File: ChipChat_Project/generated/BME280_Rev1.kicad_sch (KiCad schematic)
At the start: 0 parts

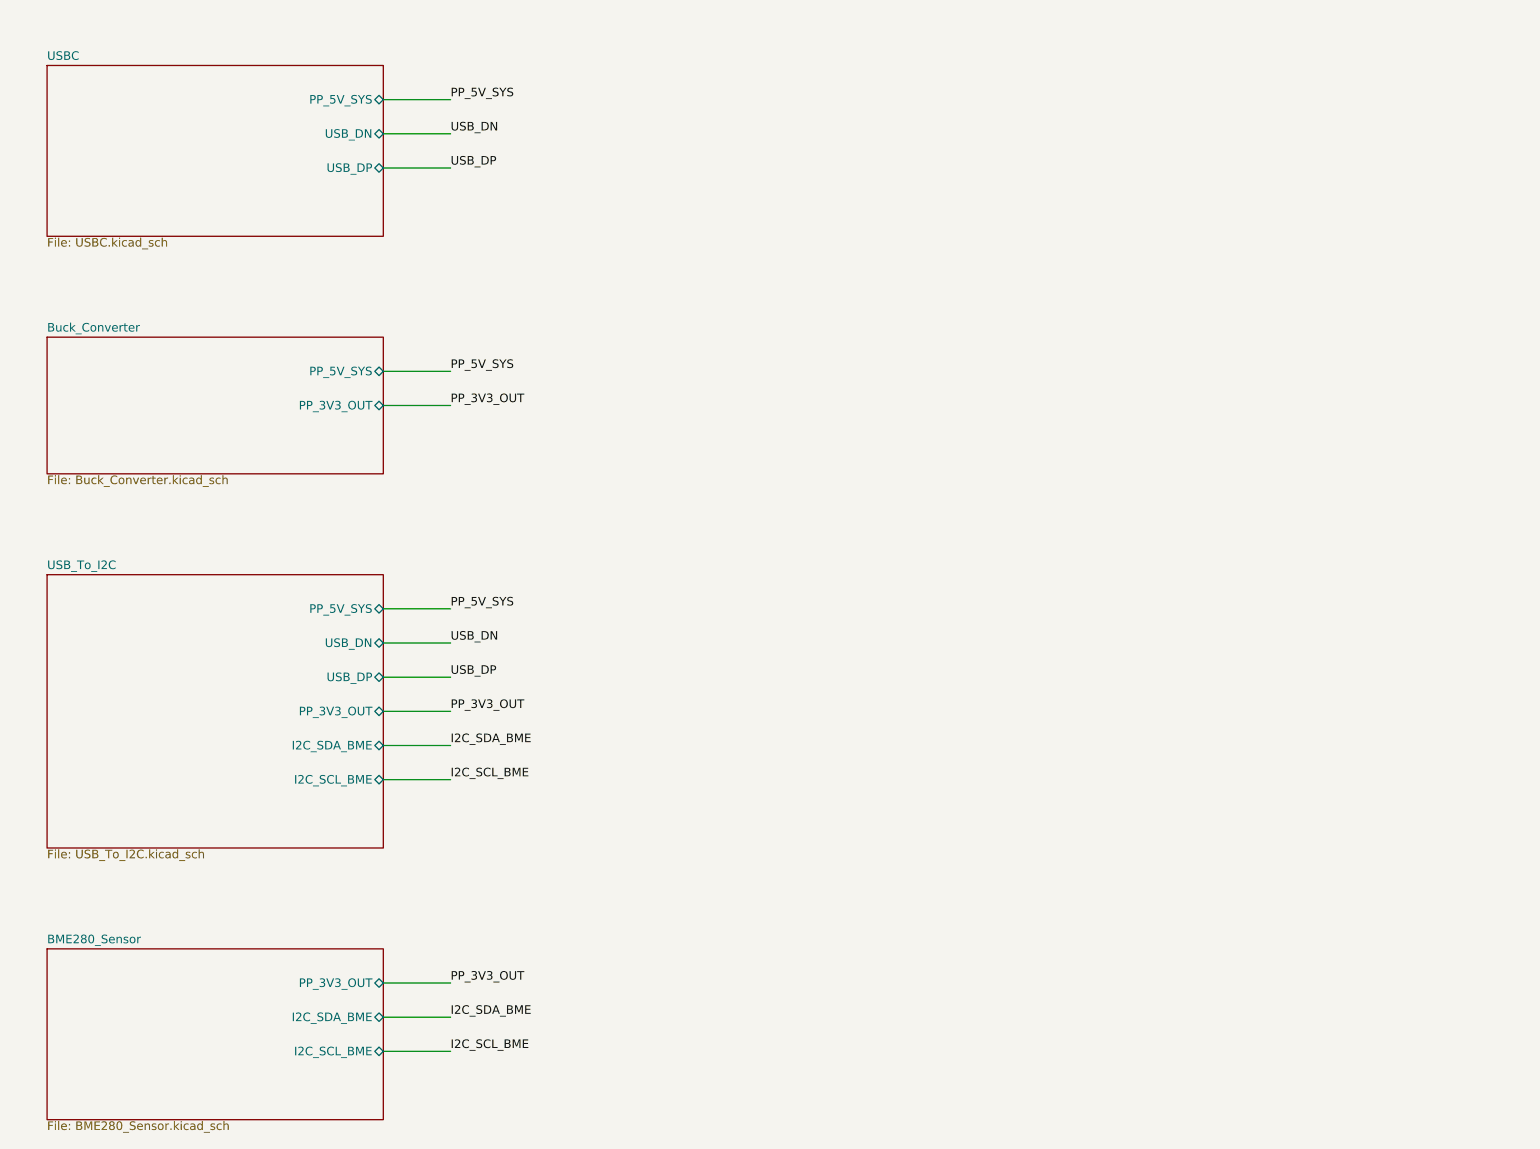
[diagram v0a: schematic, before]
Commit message: 💾 snapshot 2026-02-23_00-19-22
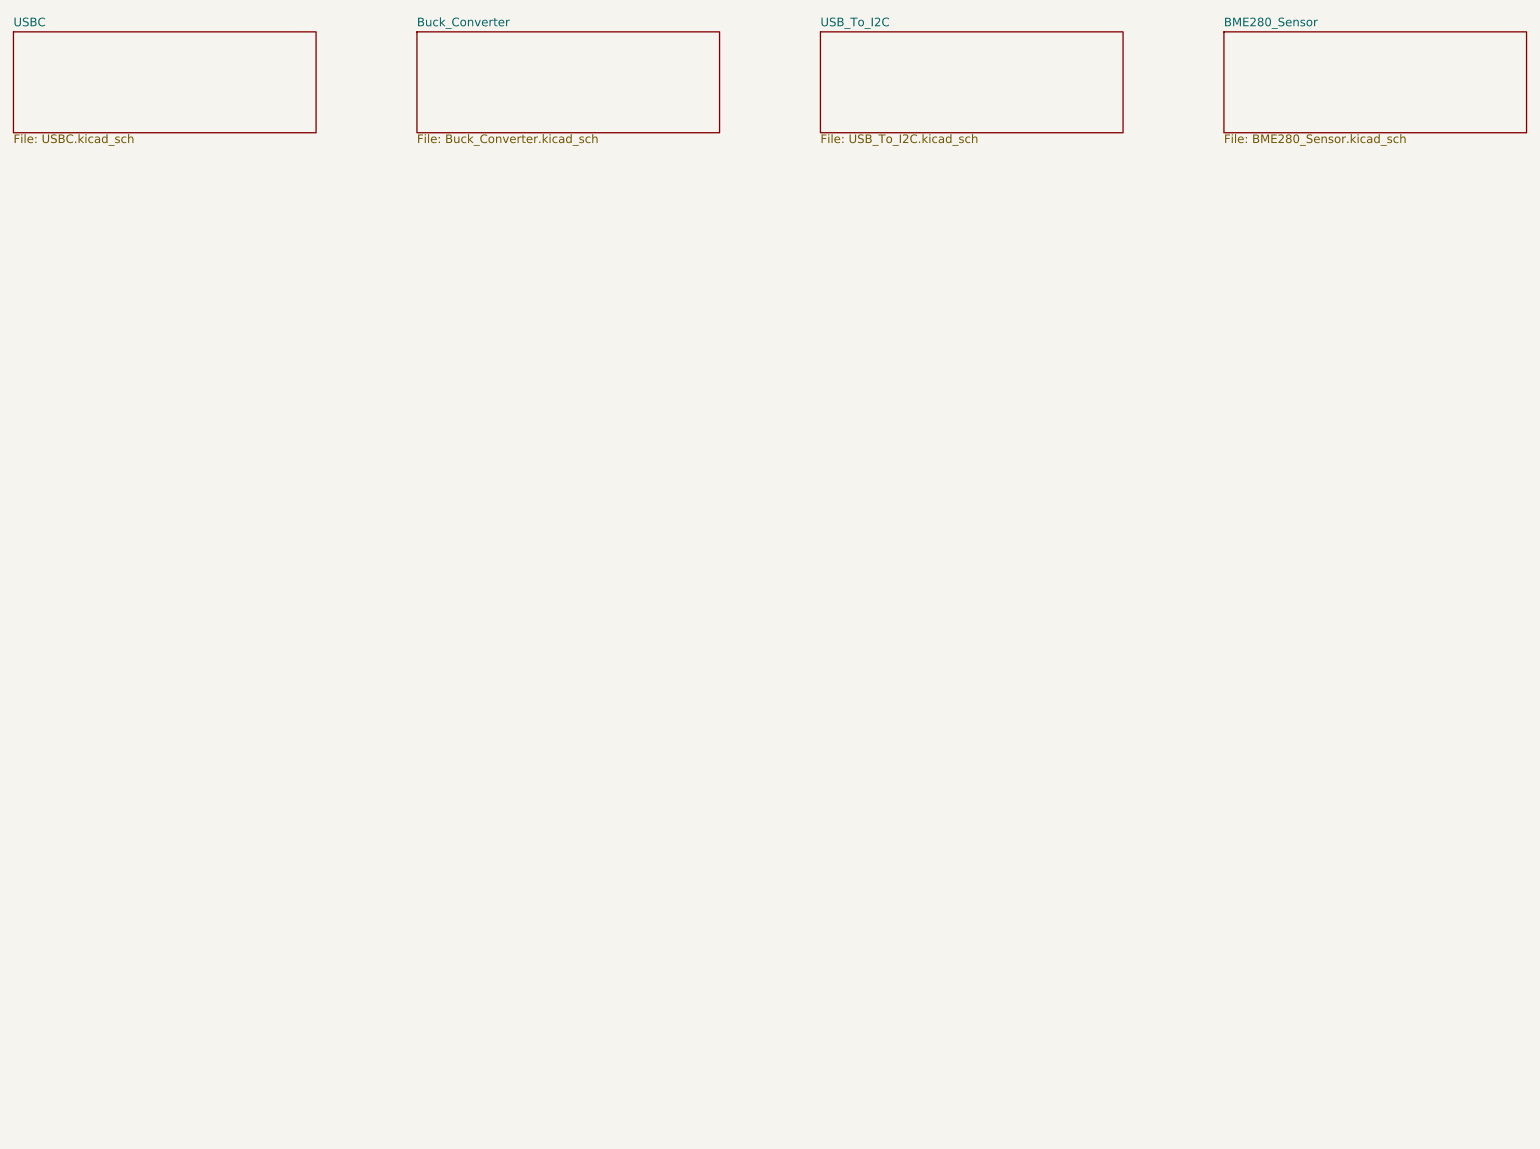
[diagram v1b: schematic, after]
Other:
- sheet BME280_Sensor ports: added none; removed I2C_SCL_BME, I2C_SDA_BME, PP_3V3_OUT
- sheet Buck_Converter ports: added none; removed PP_3V3_OUT, PP_5V_SYS
- sheet USBC ports: added none; removed PP_5V_SYS, USB_DN, USB_DP
- sheet USB_To_I2C ports: added none; removed I2C_SCL_BME, I2C_SDA_BME, PP_3V3_OUT, PP_5V_SYS, USB_DN, USB_DP
